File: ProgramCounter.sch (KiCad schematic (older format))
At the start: 6 parts, among them U13 74LS245, U14 74LS245, U15 74LS161, U16 74LS161, U17 74LS161, U18 74LS161

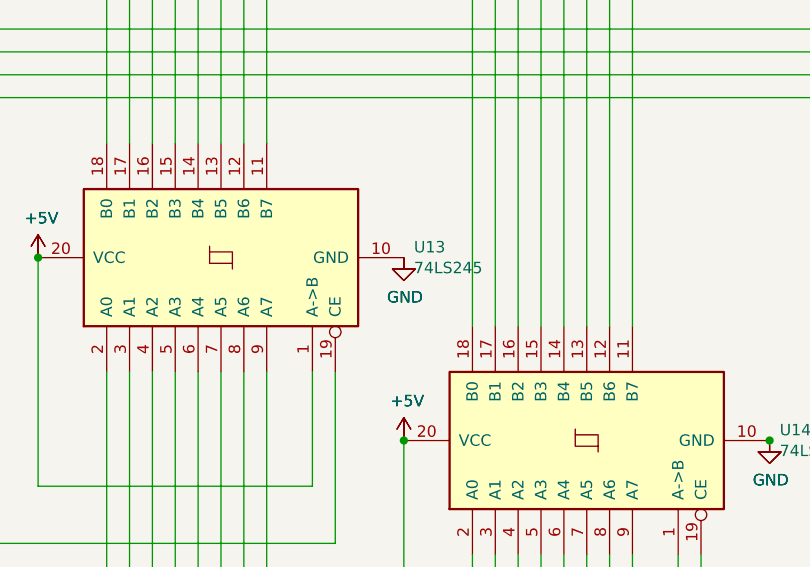
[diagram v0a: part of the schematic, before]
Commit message: fixed more errors
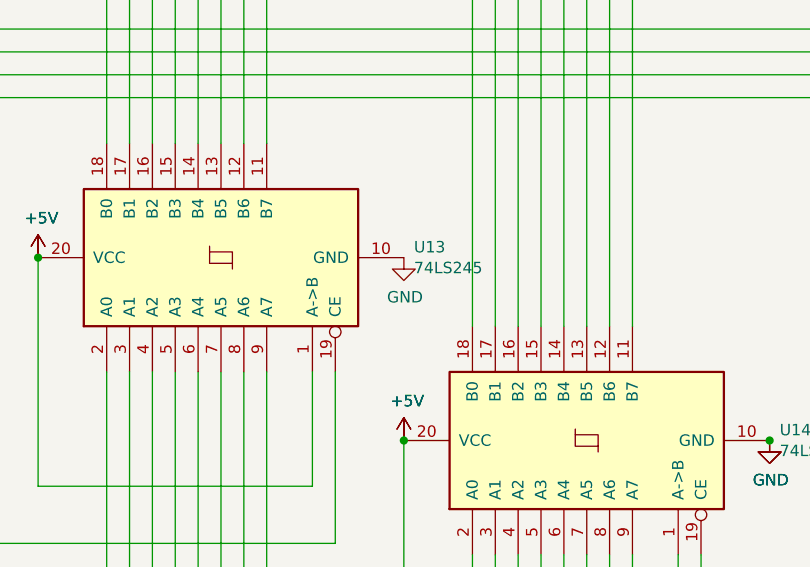
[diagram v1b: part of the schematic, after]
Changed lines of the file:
@@
-$EndComp
-$Comp
-L 16bitCpu-rescue:GND-power #PWR?
-U 1 1 5F6D5FE4
-P 3150 3650
-AR Path="/5F6D5FE4" Ref="#PWR?"  Part="1"
-AR Path="/5F67C726/5F6D5FE4" Ref="#PWR?"  Part="1"
-AR Path="/5F70885A/5F6D5FE4" Ref="#PWR?"  Part="1"
-AR Path="/5F733C5E/5F6D5FE4" Ref="#PWR?"  Part="1"
-AR Path="/602D4838/5F6D5FE4" Ref="#PWR?"  Part="1"
-AR Path="/603B00C8/5F6D5FE4" Ref="#PWR?"  Part="1"
-AR Path="/603B766D/5F6D5FE4" Ref="#PWR?"  Part="1"
-AR Path="/5F74778C/5F6D5FE4" Ref="#PWR?"  Part="1"
-AR Path="/5F6ACD14/5F6D5FE4" Ref="#PWR068"  Part="1"
-F 0 "#PWR068" H 3150 3400 50  0001 C CNN
-F 1 "GND" H 3155 3477 50  0000 C CNN
-F 2 "" H 3150 3650 50  0001 C CNN
-F 3 "" H 3150 3650 50  0001 C CNN
-	1    3150 3650
-	1    0    0    -1
 $EndComp
 $Comp
